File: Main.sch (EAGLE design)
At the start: 27 parts, among them U1 L298, U2 LM 1084 IT5,0, U3 LM 1084 IT3,3, U4 L298, X1 12V

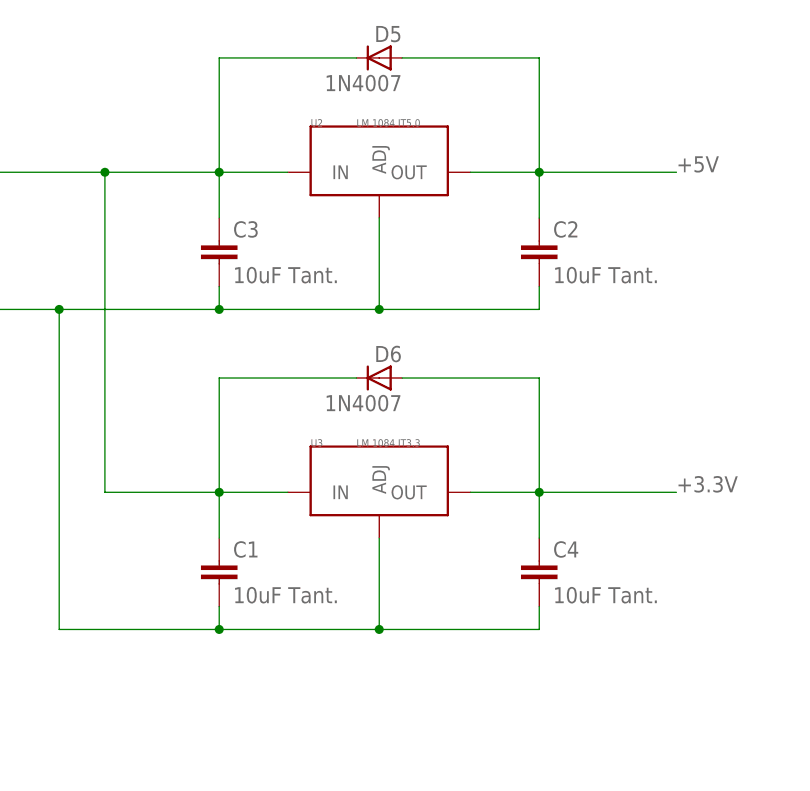
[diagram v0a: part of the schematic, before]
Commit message: some routing experiments
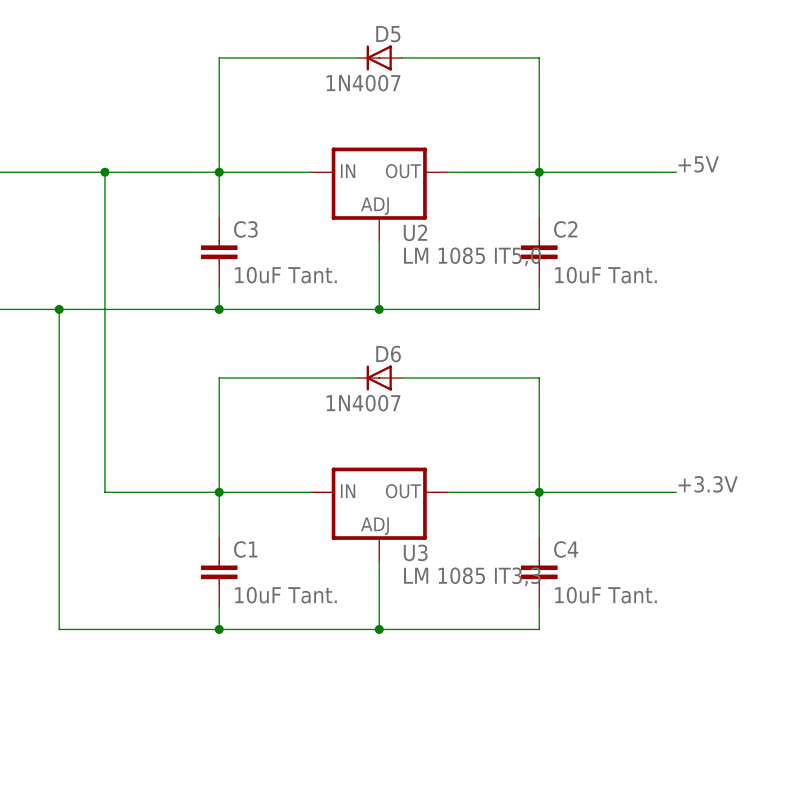
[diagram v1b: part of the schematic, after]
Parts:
- U2: value LM 1084 IT5,0 -> LM 1085 IT5,0; device PP_PowerIC:LM1084TO-263-3 -> linear-technology-3:LT1085IT-V
- U3: value LM 1084 IT3,3 -> LM 1085 IT3,3; device PP_PowerIC:LM1084TO-263-3 -> linear-technology-3:LT1085IT-V
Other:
- moved on the sheet: U2, U3
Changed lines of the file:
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@@
 <layer number="223" name="223bmp" color="24" fill="1" visible="no" active="no"/>
 <layer number="224" name="224bmp" color="25" fill="1" visible="no" active="no"/>
+<layer number="231" name="Eagle3D_PG1" color="14" fill="1" visible="yes" active="yes"/>
+<layer number="232" name="Eagle3D_PG2" color="14" fill="2" visible="yes" active="yes"/>
+<layer number="233" name="Eagle3D_PG3" color="14" fill="4" visible="yes" active="yes"/>
 <layer number="250" name="Descript" color="3" fill="1" visible="no" active="no"/>
 <layer number="251" name="SMDround" color="12" fill="11" visible="no" active="no"/>
@@
 </classes>
 <parts>
-<part name="U2" library="PP_PowerIC" deviceset="LM1084" device="TO-263-3" value="LM 1084 IT5,0"/>
+<part name="U2" library="linear-technology-3" deviceset="LT1085*" device="T-V" technology="I" value="LM 1085 IT5,0"/>
 <part name="D5" library="semicon-smd-ipc" deviceset="D-" device="MLL-41" value="1N4007"/>
 <part name="C1" library="rcl" deviceset="C-EU" device="025-040X050" value="10uF Tant."/>
 <part name="C2" library="rcl" deviceset="C-EU" device="025-040X050" value="10uF Tant."/>
 <part name="X1" library="con-wago-508" deviceset="W237-02P" device="" value="12V"/>
-<part name="U3" library="PP_PowerIC" deviceset="LM1084" device="TO-263-3" value="LM 1084 IT3,3"/>
+<part name="U3" library="linear-technology-3" deviceset="LT1085*" device="T-V" technology="I" value="LM 1085 IT3,3"/>
 <part name="D6" library="semicon-smd-ipc" deviceset="D-" device="MLL-41" value="1N4007"/>
 <part name="C4" library="rcl" deviceset="C-EU" device="025-040X050" value="10uF Tant."/>
@@
 <label x="-378.46" y="340.36" size="1.778" layer="95"/>
 <pinref part="U2" gate="G$1" pin="OUT"/>
-<wire x1="-393.7" y1="340.36" x2="-401.32" y2="340.36" width="0.1524" layer="91"/>
+<wire x1="-393.7" y1="340.36" x2="-403.86" y2="340.36" width="0.1524" layer="91"/>
 </segment>
 <segment>
@@
 <label x="-378.46" y="304.8" size="1.778" layer="95"/>
 <pinref part="U3" gate="G$1" pin="OUT"/>
-<wire x1="-401.32" y1="304.8" x2="-393.7" y2="304.8" width="0.1524" layer="91"/>
+<wire x1="-403.86" y1="304.8" x2="-393.7" y2="304.8" width="0.1524" layer="91"/>
 </segment>
 </net>
 <net name="+12V" class="0">
 <segment>
-<wire x1="-429.26" y1="304.8" x2="-421.64" y2="304.8" width="0.1524" layer="91"/>
+<wire x1="-429.26" y1="304.8" x2="-419.1" y2="304.8" width="0.1524" layer="91"/>
 <junction x="-429.26" y="304.8"/>
 <wire x1="-429.26" y1="304.8" x2="-429.26" y2="317.5" width="0.1524" layer="91"/>
@@
 <pinref part="U3" gate="G$1" pin="IN"/>
 <wire x1="-429.26" y1="304.8" x2="-441.96" y2="304.8" width="0.1524" layer="91"/>
-<wire x1="-429.26" y1="340.36" x2="-421.64" y2="340.36" width="0.1524" layer="91"/>
+<wire x1="-429.26" y1="340.36" x2="-419.1" y2="340.36" width="0.1524" layer="91"/>
 <junction x="-429.26" y="340.36"/>
 <wire x1="-429.26" y1="340.36" x2="-429.26" y2="353.06" width="0.1524" layer="91"/>
@@
 <wire x1="-411.48" y1="289.56" x2="-393.7" y2="289.56" width="0.1524" layer="91"/>
 <pinref part="U3" gate="G$1" pin="ADJ"/>
-<wire x1="-411.48" y1="299.72" x2="-411.48" y2="289.56" width="0.1524" layer="91"/>
+<wire x1="-411.48" y1="297.18" x2="-411.48" y2="289.56" width="0.1524" layer="91"/>
 <junction x="-411.48" y="289.56"/>
 <wire x1="-411.48" y1="325.12" x2="-393.7" y2="325.12" width="0.1524" layer="91"/>
 <pinref part="U2" gate="G$1" pin="ADJ"/>
-<wire x1="-411.48" y1="335.28" x2="-411.48" y2="325.12" width="0.1524" layer="91"/>
+<wire x1="-411.48" y1="332.74" x2="-411.48" y2="325.12" width="0.1524" layer="91"/>
 <junction x="-411.48" y="325.12"/>
 <wire x1="-447.04" y1="325.12" x2="-429.26" y2="325.12" width="0.1524" layer="91"/>
